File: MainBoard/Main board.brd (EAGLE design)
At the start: 100 x 80 mm, 9 parts

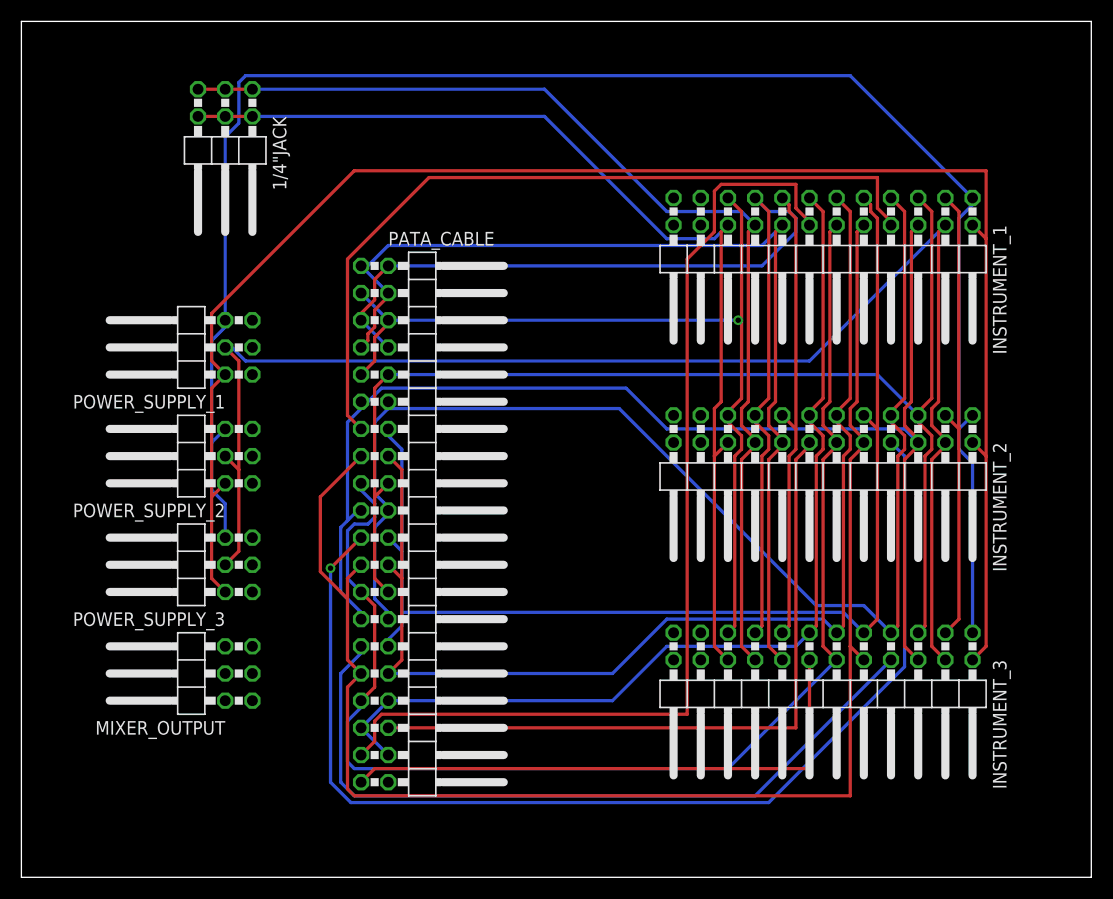
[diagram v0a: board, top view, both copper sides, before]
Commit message: Update Main board.brd
Version 2
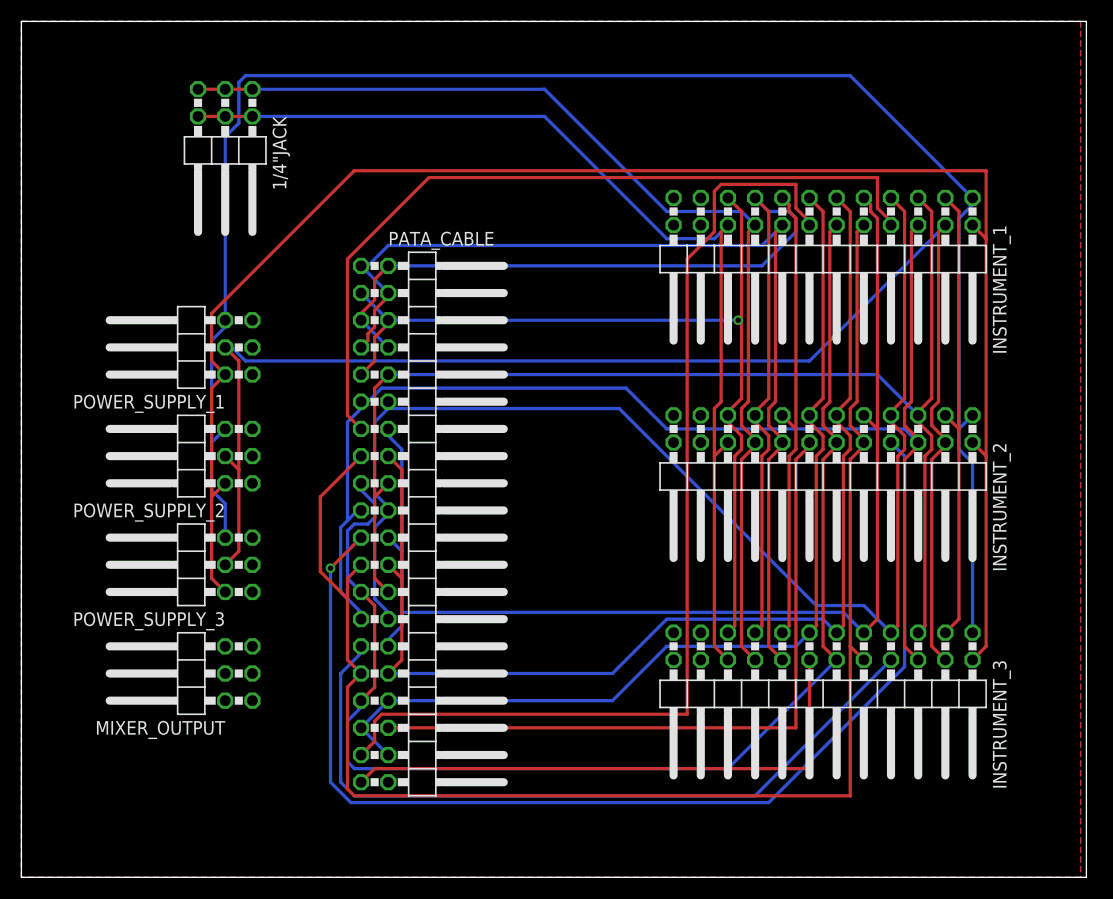
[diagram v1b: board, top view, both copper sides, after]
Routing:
- added copper zone on layer 1, net GND
- added copper zone on layer 16, net GND
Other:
- board size 100 x 80 mm -> 99.5 x 80 mm
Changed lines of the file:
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@@
 <setting verticaltext="up"/>
 </settings>
-<grid distance="50" unitdist="mil" unit="inch" style="dots" multiple="1" display="yes" altdistance="5" altunitdist="mil" altunit="inch"/>
+<grid distance="1" unitdist="mm" unit="mm" style="lines" multiple="1" display="yes" altdistance="0.025" altunitdist="inch" altunit="inch"/>
 <layers>
 <layer number="1" name="Top" color="4" fill="1" visible="yes" active="yes"/>
@@
 <layer number="19" name="Unrouted" color="6" fill="1" visible="yes" active="yes"/>
 <layer number="20" name="Dimension" color="24" fill="1" visible="yes" active="yes"/>
-<layer number="21" name="tPlace" color="7" fill="1" visible="yes" active="yes"/>
-<layer number="22" name="bPlace" color="7" fill="1" visible="yes" active="yes"/>
+<layer number="21" name="tPlace" color="16" fill="1" visible="yes" active="yes"/>
+<layer number="22" name="bPlace" color="16" fill="1" visible="yes" active="yes"/>
 <layer number="23" name="tOrigins" color="15" fill="1" visible="yes" active="yes"/>
 <layer number="24" name="bOrigins" color="15" fill="1" visible="yes" active="yes"/>
 <layer number="25" name="tNames" color="7" fill="1" visible="yes" active="yes"/>
-<layer number="26" name="bNames" color="7" fill="1" visible="yes" active="yes"/>
-<layer number="27" name="tValues" color="7" fill="1" visible="yes" active="yes"/>
-<layer number="28" name="bValues" color="7" fill="1" visible="yes" active="yes"/>
+<layer number="26" name="bNames" color="16" fill="1" visible="yes" active="yes"/>
+<layer number="27" name="tValues" color="16" fill="1" visible="no" active="yes"/>
+<layer number="28" name="bValues" color="16" fill="1" visible="no" active="yes"/>
 <layer number="29" name="tStop" color="7" fill="3" visible="no" active="yes"/>
 <layer number="30" name="bStop" color="7" fill="6" visible="no" active="yes"/>
@@
 <layer number="49" name="Reference" color="7" fill="1" visible="yes" active="yes"/>
 <layer number="50" name="dxf" color="7" fill="1" visible="no" active="no"/>
-<layer number="51" name="tDocu" color="7" fill="1" visible="yes" active="yes"/>
-<layer number="52" name="bDocu" color="7" fill="1" visible="yes" active="yes"/>
+<layer number="51" name="tDocu" color="16" fill="1" visible="yes" active="yes"/>
+<layer number="52" name="bDocu" color="16" fill="1" visible="yes" active="yes"/>
 <layer number="53" name="tGND_GNDA" color="7" fill="9" visible="no" active="no"/>
 <layer number="54" name="bGND_GNDA" color="1" fill="9" visible="no" active="no"/>
@@
 <board>
 <plain>
-<wire x1="0" y1="0" x2="100" y2="0" width="0" layer="20"/>
-<wire x1="100" y1="0" x2="100" y2="80" width="0" layer="20"/>
-<wire x1="100" y1="80" x2="0" y2="80" width="0" layer="20"/>
+<wire x1="0" y1="0" x2="99.54" y2="0" width="0" layer="20"/>
+<wire x1="99.54" y1="0" x2="99.54" y2="80" width="0" layer="20"/>
+<wire x1="99.54" y1="80" x2="0" y2="80" width="0" layer="20"/>
 <wire x1="0" y1="80" x2="0" y2="0" width="0" layer="20"/>
 </plain>
@@
 <wire x1="81.28" y1="20.32" x2="68.58" y2="7.62" width="0.3048" layer="16"/>
 </signal>
+<signal name="GND">
+<polygon width="0.1524" layer="1">
+<vertex x="0" y="0"/>
+<vertex x="0" y="80"/>
+<vertex x="99" y="80"/>
+<vertex x="99" y="0"/>
+</polygon>
+<polygon width="0.1524" layer="16">
+<vertex x="0" y="0"/>
+<vertex x="0" y="80"/>
+<vertex x="99" y="80"/>
+<vertex x="99" y="0"/>
+</polygon>
+</signal>
 </signals>
